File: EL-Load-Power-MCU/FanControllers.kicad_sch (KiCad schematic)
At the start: 28 parts, among them J5 PN sensor, J6 PN sensor, M1 Fan_4pin, M2 Fan_4pin, M3 Fan_4pin, U1 MAX31760, U3 MAX31760

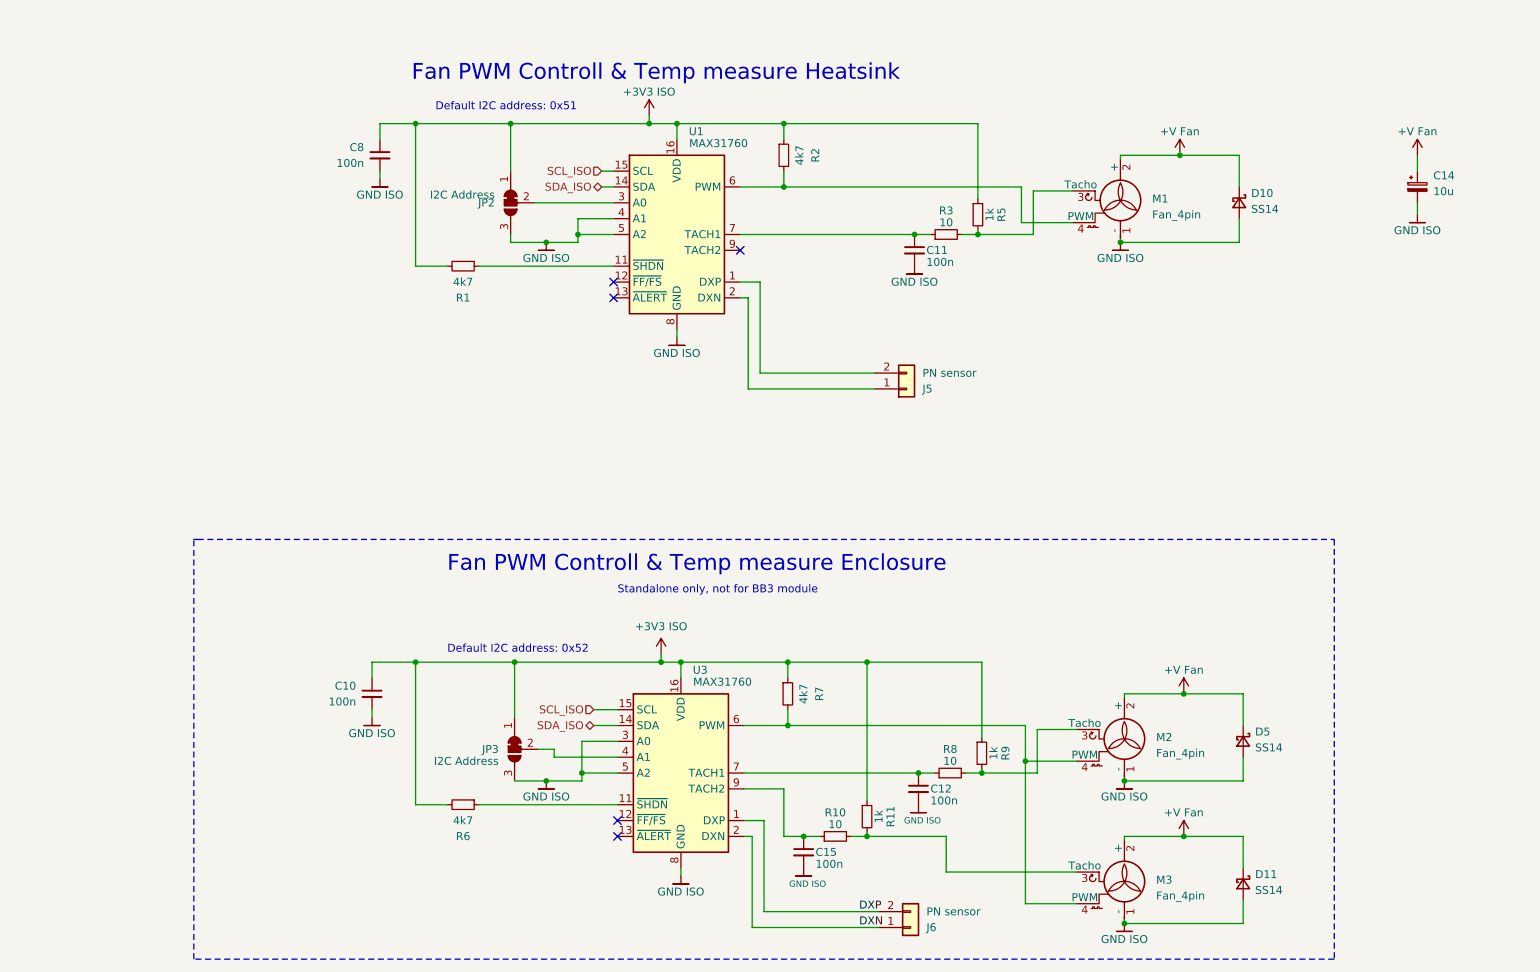
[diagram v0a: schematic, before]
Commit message: EL-Load-Power-MCU PCB v4r4 release.
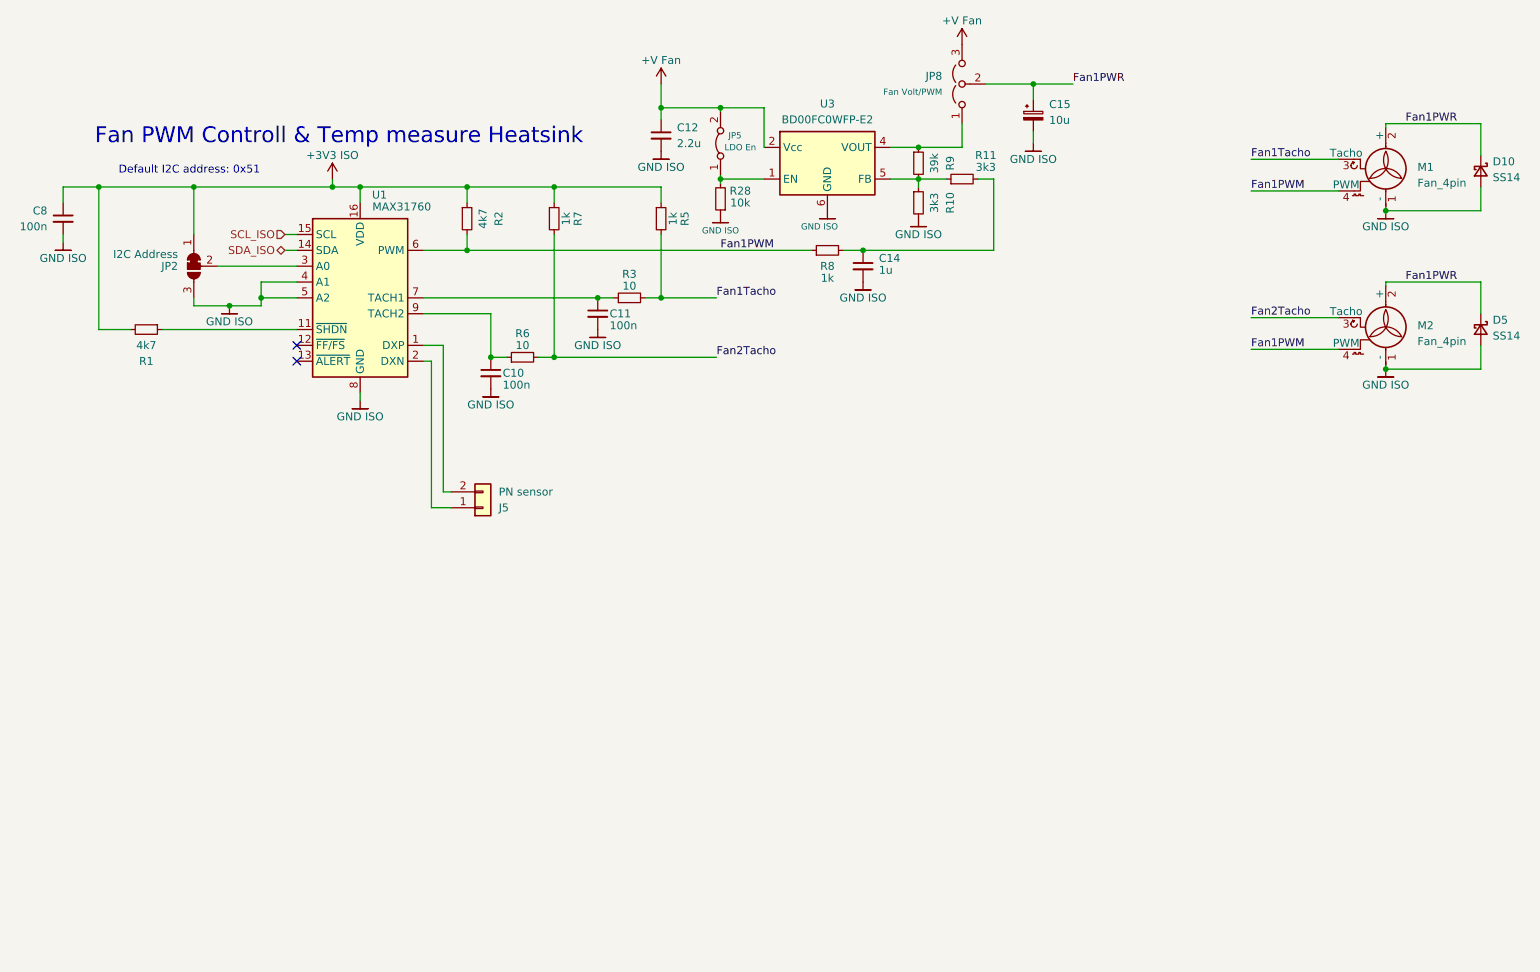
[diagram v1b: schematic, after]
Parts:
- removed C14: 10u, Capacitor_SMD:CP_Elec_6.3x5.8, symbol Device:C_Polarized_Small
- removed C15: 100n, Capacitor_SMD:C_0805_2012Metric, symbol Device:C_Small
- removed D11: SS14, Diode_SMD:D_SMA, symbol Device:D_Schottky_Small
- removed J6: PN sensor, Connector_PinHeader_2.54mm:PinHeader_1x02_P2.54mm_Vertical, symbol Connector_Generic:Conn_01x02
- removed JP3: I2C Address, Jumper:SolderJumper-3_P1.3mm_Bridged2Bar12_RoundedPad1.0x1.5mm, symbol Jumper:SolderJumper_3_Bridged12
- removed M3: Fan_4pin, Connector:FanPinHeader_1x04_P2.54mm_Vertical, symbol Motor:Fan_4pin
- removed U3: MAX31760, Package_SO:QSOP-16_3.9x4.9mm_P0.635mm, symbol EL-Load:MAX31760
- added C14: 1u, Capacitor_SMD:C_0805_2012Metric, symbol Device:C_Small
- added C15: 10u, Capacitor_SMD:CP_Elec_5x5.8, symbol Device:C_Polarized_Small
- added JP5: LDO En, Connector_PinHeader_2.54mm:PinHeader_1x02_P2.54mm_Vertical, symbol Jumper:Jumper_2_Bridged
- added JP8: Fan Volt/PWM, Connector_PinHeader_2.54mm:PinHeader_1x03_P2.54mm_Vertical, symbol Jumper:Jumper_3_Open
- added R28: 10k, Resistor_SMD:R_0805_2012Metric, symbol Device:R_Small
- added U3: BD00FC0WFP-E2, Package_TO_SOT_SMD:TO-252-5_TabPin6, symbol EL-Load:BD00FC0W
- C10, C11, C8: Part_Name C_100.0nF_50V_0805_10% -> C_100.0nF_50V_0805_10%_X7R
- C12: value 100n -> 2.2u; Part_Name C_100.0nF_50V_0805_10% -> C_2.2uF_25V_X7R_10%_0805
- R1, R2, R3, R5: footprint Resistor_SMD:R_0805_2012Metric_Pad1.20x1.40mm_HandSolder -> Resistor_SMD:R_0805_2012Metric
- R10: value 10 -> 3k3; footprint Resistor_SMD:R_0805_2012Metric_Pad1.20x1.40mm_HandSolder -> Resistor_SMD:R_0805_2012Metric; Part_Name R_10.0Ω_0805_1% -> R_3.3kΩ_0805_1%
- R11: value 1k -> 3k3; footprint Resistor_SMD:R_0805_2012Metric_Pad1.20x1.40mm_HandSolder -> Resistor_SMD:R_0805_2012Metric; Part_Name R_1.0kΩ_0805_1% -> R_3.3kΩ_0805_1%
- R6: value 4k7 -> 10; footprint Resistor_SMD:R_0805_2012Metric_Pad1.20x1.40mm_HandSolder -> Resistor_SMD:R_0805_2012Metric; Part_Name R_4.7kΩ_0805_1% -> R_10.0Ω_0805_1%
- R7: value 4k7 -> 1k; footprint Resistor_SMD:R_0805_2012Metric_Pad1.20x1.40mm_HandSolder -> Resistor_SMD:R_0805_2012Metric; Part_Name R_4.7kΩ_0805_1% -> R_1.0kΩ_0805_1%
- R8: value 10 -> 1k; footprint Resistor_SMD:R_0805_2012Metric_Pad1.20x1.40mm_HandSolder -> Resistor_SMD:R_0805_2012Metric; Part_Name R_10.0Ω_0805_1% -> R_1.0kΩ_0805_1%
- R9: value 1k -> 39k; footprint Resistor_SMD:R_0805_2012Metric_Pad1.20x1.40mm_HandSolder -> Resistor_SMD:R_0805_2012Metric; Part_Name R_1.0kΩ_0805_1% -> R_39.0kΩ_0805_1%
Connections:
- net +3V3_ISO: no longer C10.1, R11.1, R6.2, R9.1
- net +V_FANS: now also C12.1, JP5.2 (B), JP8.3 (B), U3.2 (Vcc); no longer D10.1 (K), D5.1 (K), M1.2 (+), M2.2 (+)
- net GND_ISO: now also R10.2, C14.2, C15.2, R28.1, U3.6 (GND)
- net Fan1PWM: now reaches R8.1
- net Fan1PWM: now also M1.4 (PWM), M2.4 (PWM), R2.2, U1.6 (PWM); no longer C12.1
- net Fan2Tacho: now reaches R7.2
- net Fan2Tacho: now also M2.3 (Tacho), R6.2; no longer M2.4 (PWM)
- net at R6.1: now also C10.1, U1.9 (TACH2)
- net at R11.2: now also R8.2, C14.1; no longer R10.2
- net at R10.1: now also R11.1, R9.2, U3.5 (FB)
- net Fan1Tacho: now reaches M1.3 (Tacho), R3.2, R5.2
- new net: JP5.1 (A), R28.2, U3.1 (EN)
- new net: JP8.1 (A), R9.1, U3.4 (VOUT)
- new net Fan1PWR: C15.1, D10.1 (K), D5.1 (K), JP8.2 (C), M1.2 (+), M2.2 (+)
- no-connect marks 5 -> 2
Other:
- note removed: "Default I2C address: 0x52"
- note removed: "Fan PWM Controll & Temp measure Enclosure"
- note removed: "Standalone only, not for BB3 module"
- moved on the sheet: C11, C8, D10, J5, JP2, M1, R1, R2, R3, R5, U1
